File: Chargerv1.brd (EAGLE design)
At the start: 25.4 x 93.7 mm, 12 parts, among them J1 POWER_JACKPTH_LOCK, U1 MCP73831, X1 USB-MICROB

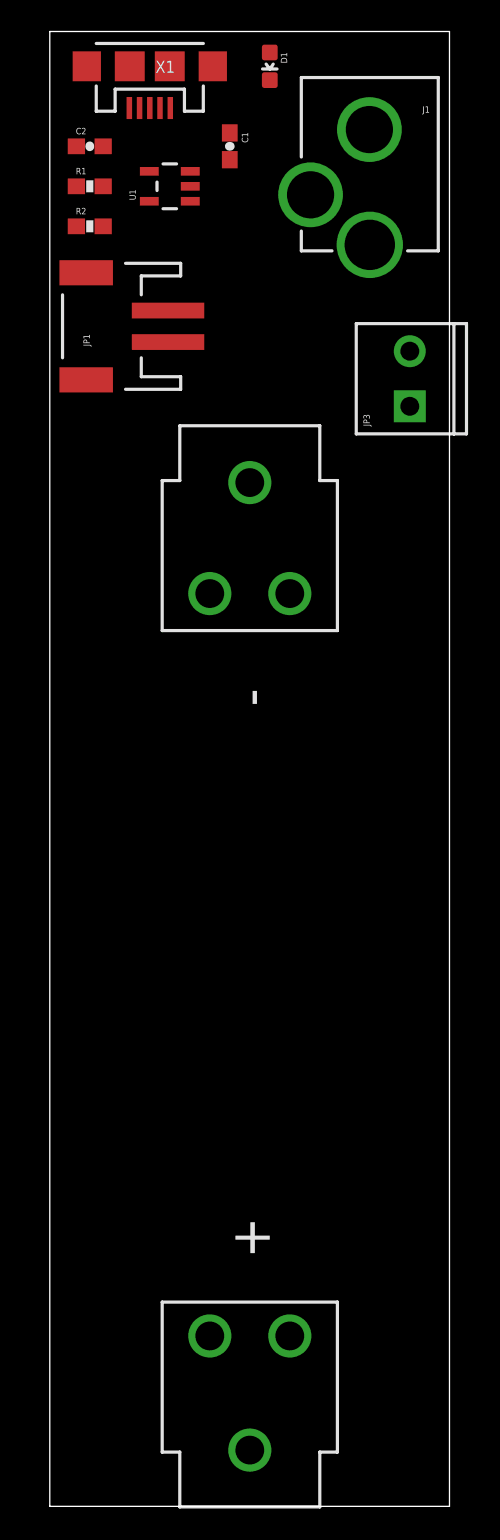
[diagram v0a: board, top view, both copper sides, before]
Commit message: Routed Board
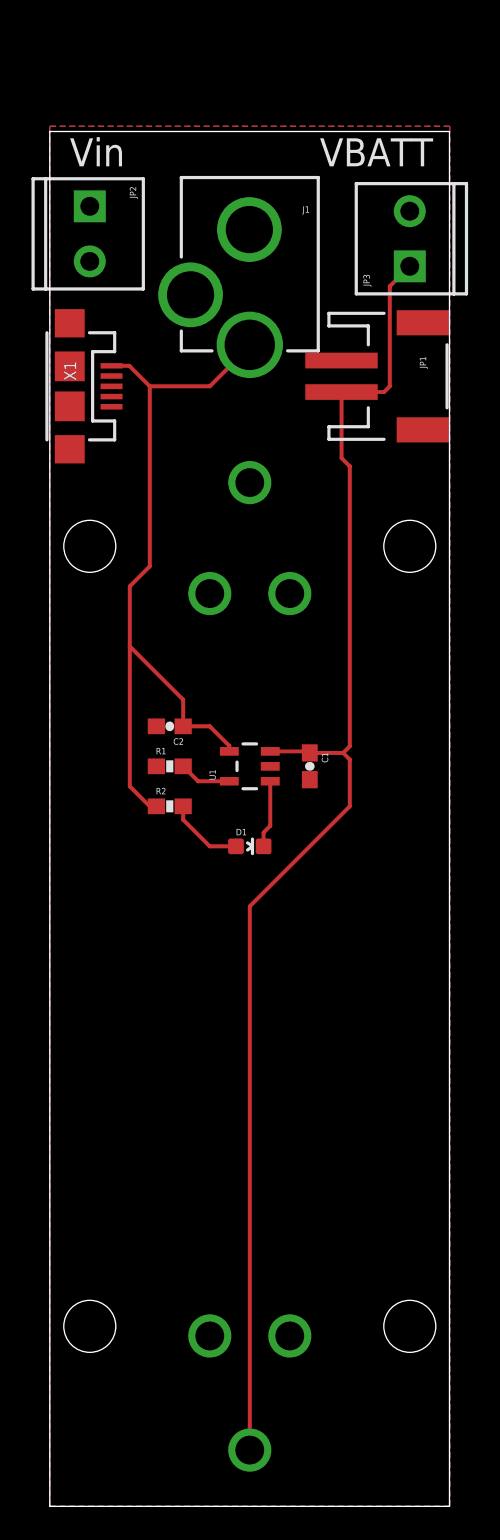
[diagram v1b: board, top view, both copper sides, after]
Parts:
- added JP2: M023.5MM, SparkFun-Connectors:SCREWTERMINAL-3.5MM-2
- added STANDOFF1, STANDOFF2, STANDOFF3, STANDOFF4: STAND-OFF, SparkFun-Electromechanical:STAND-OFF
- moved D1 49.5 mm to (12.7, 41.9), turned to 270 degrees
- moved C1 39.7 mm to (16.5, 47.0)
- moved C2 37.2 mm to (7.62, 49.5), turned to 180 degrees
- moved R2 37.2 mm to (7.62, 44.5)
- moved R1 37.2 mm to (7.62, 47.0)
- moved U1 37.2 mm to (12.7, 47.0)
- moved X1 20.9 mm to (1.27, 71.1), turned to 270 degrees
- moved JP1 18.7 mm to (22.2, 71.8), turned to 270 degrees
- moved J1 9.92 mm to (12.7, 87.6)
- moved JP3 8.89 mm to (22.9, 78.7)
- flipped B1 to the bottom
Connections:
- net 5V: now also JP2.1
- net GND: now also JP2.2
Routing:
- net V_BATT: track 0.00 -> 86.4 mm
- net 5V: track 0.00 -> 48.9 mm
- net N$1: track 0.00 -> 4.90 mm
- net N$2: track 0.00 -> 4.31 mm
- net N$7: track 0.00 -> 3.32 mm
- added copper zone on layer 16, net 5V
- added copper zone on layer 1, net GND
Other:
- board size 25.4 x 93.7 mm -> 25.4 x 87.3 mm
- board text added: "+"
- board text added: "-"
- board text added: "Single Cell Lipo Charger"
- board text added: "VBATT"
- board text added: "Vin"
